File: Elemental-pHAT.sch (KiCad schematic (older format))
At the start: 7 parts

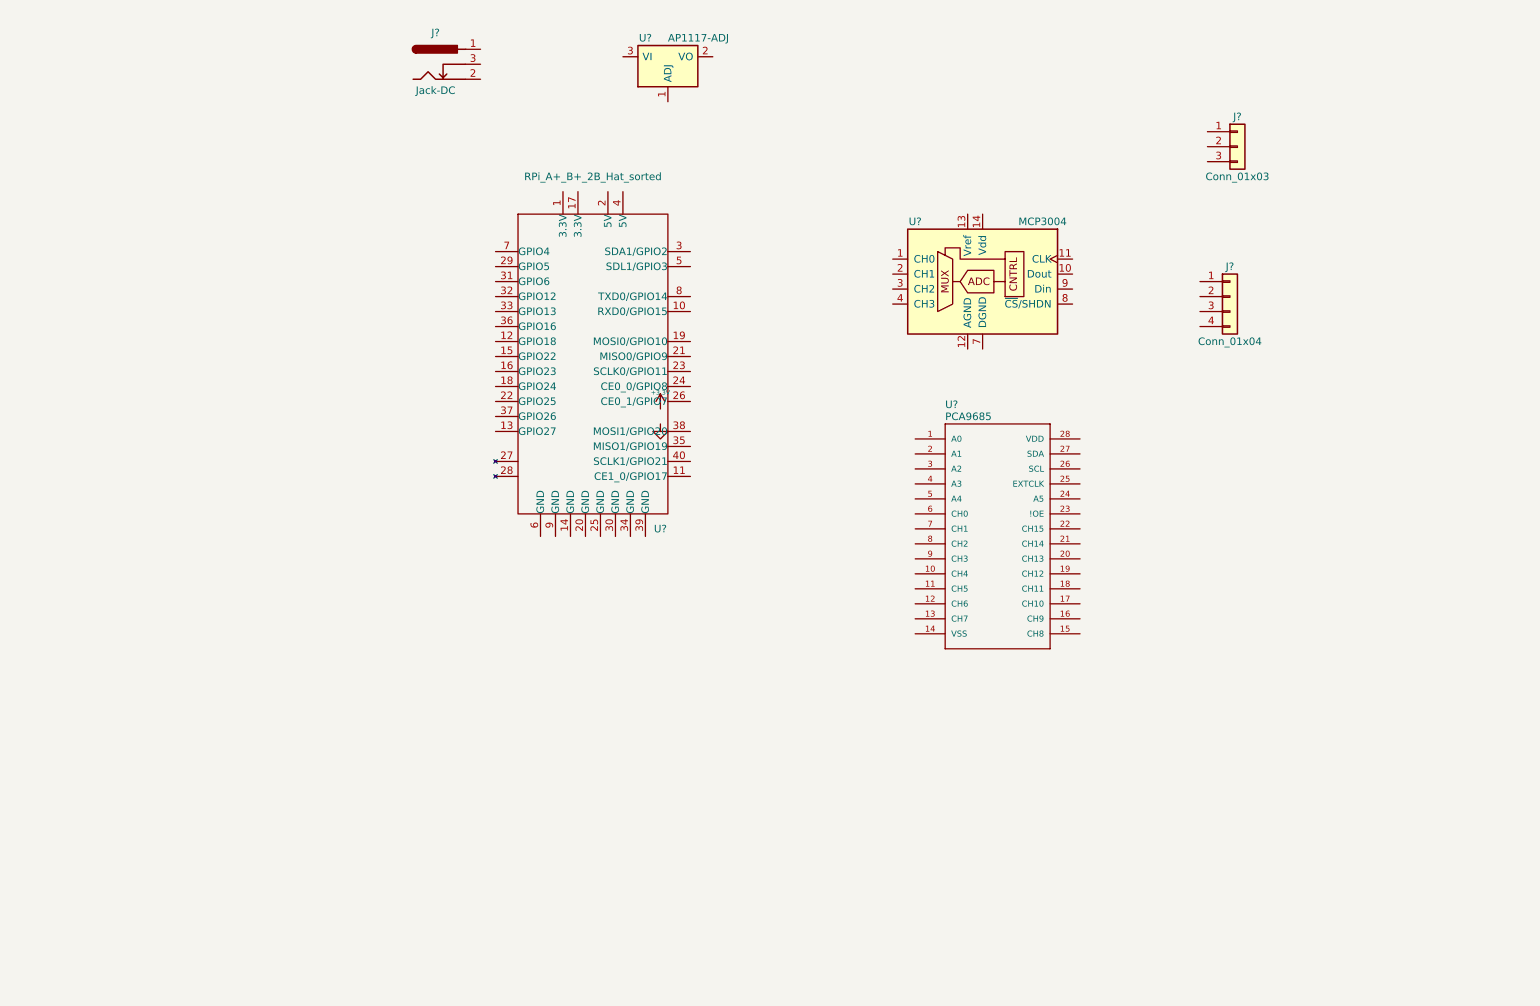
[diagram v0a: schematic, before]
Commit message: conectores añadidos
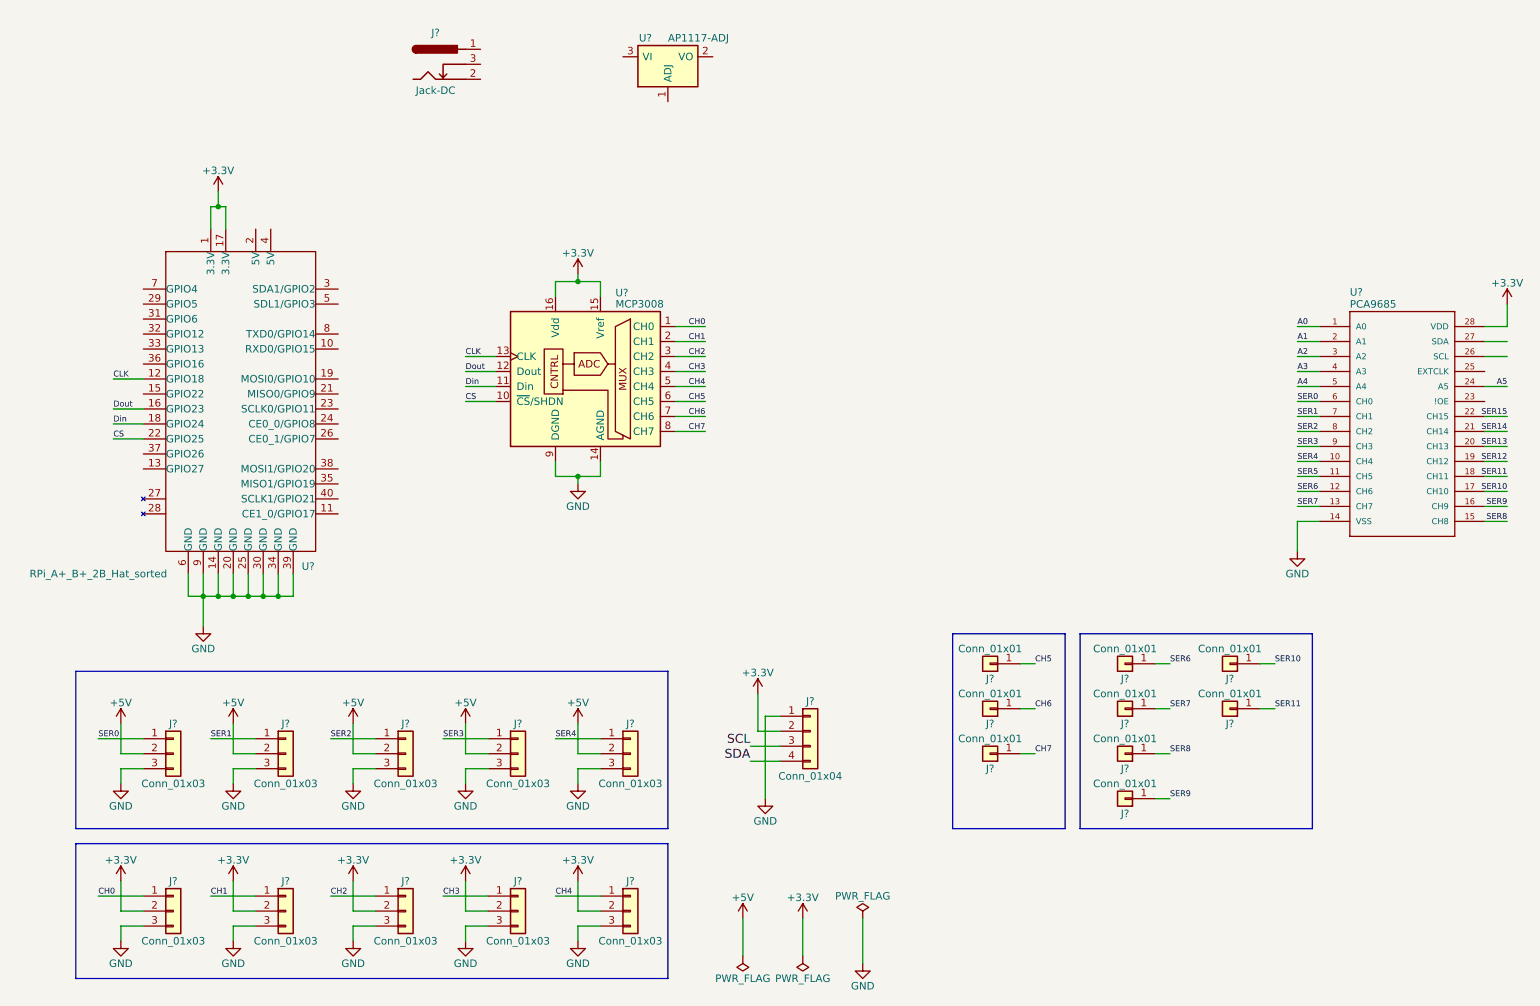
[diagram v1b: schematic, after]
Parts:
- removed U?: MCP3004, symbol MCP3004
- added J? (x9): Conn_01x03, symbol Conn_01x03
- added J? (x9): Conn_01x01, symbol Conn_01x01
- added U?: MCP3008, symbol MCP3008
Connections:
- net +3V3: now also J?.2 (Pin_2), J?.2 (Pin_2), U?.1 (3.3V), U?.17 (3.3V), U?.28 (VDD), J?.2 (Pin_2), J?.2 (Pin_2), J?.2 (Pin_2), J?.2 (Pin_2), U?.15 (Vref), U?.16 (Vdd)
- net GND: now also J?.1 (Pin_1), J?.3 (Pin_3), U?.14 (GND), U?.14 (VSS), U?.20 (GND), U?.25 (GND), U?.30 (GND), U?.34 (GND), U?.39 (GND), U?.6 (GND), U?.9 (GND), J?.3 (Pin_3), J?.3 (Pin_3), J?.3 (Pin_3), J?.3 (Pin_3), J?.3 (Pin_3), J?.3 (Pin_3), J?.3 (Pin_3), J?.3 (Pin_3), J?.3 (Pin_3), U?.14 (AGND), U?.9 (DGND)
- net CLK: now reaches U?.12 (GPIO18)
- net CLK: now also U?.13 (CLK)
- net Dout: now reaches U?.16 (GPIO23)
- net Dout: now also U?.12 (Dout)
- net Din: now reaches U?.18 (GPIO24)
- net Din: now also U?.11 (Din)
- net CS: now reaches U?.22 (GPIO25)
- net CS: now also U?.10 (~CS~/SHDN)
- net A0: now reaches U?.1 (A0)
- net SER4: now reaches U?.10 (CH4)
- net SER4: now also J?.1 (Pin_1)
- net SER5: now reaches U?.11 (CH5)
- net SER6: now reaches U?.12 (CH6)
- net SER6: now also J?.1 (Pin_1)
- net SER7: now reaches U?.13 (CH7)
- net SER7: now also J?.1 (Pin_1)
- net SER8: now reaches U?.15 (CH8)
- net SER8: now also J?.1 (Pin_1)
- net SER9: now reaches U?.16 (CH9)
- net SER9: now also J?.1 (Pin_1)
- net SER10: now reaches U?.17 (CH10)
- net SER10: now also J?.1 (Pin_1)
- net SER11: now reaches U?.18 (CH11)
- net SER11: now also J?.1 (Pin_1)
- net SER12: now reaches U?.19 (CH12)
- net A1: now reaches U?.2 (A1)
- net SER13: now reaches U?.20 (CH13)
- net SER14: now reaches U?.21 (CH14)
- net SER15: now reaches U?.22 (CH15)
- net A5: now reaches U?.24 (A5)
- net A2: now reaches U?.3 (A2)
- net A3: now reaches U?.4 (A3)
- net A4: now reaches U?.5 (A4)
- net SER0: now reaches U?.6 (CH0)
- net SER0: now also J?.1 (Pin_1)
- net SER1: now reaches U?.7 (CH1)
- net SER1: now also J?.1 (Pin_1)
- net SER2: now reaches U?.8 (CH2)
- net SER2: now also J?.1 (Pin_1)
- net SER3: now reaches U?.9 (CH3)
- net SER3: now also J?.1 (Pin_1)
- net CH0: now reaches J?.1 (Pin_1)
- net CH0: now also U?.1 (CH0)
- net SCL: now reaches J?.3 (Pin_3)
- net SDA: now reaches J?.4 (Pin_4)
- new net +5V: J?.2 (Pin_2), J?.2 (Pin_2), J?.2 (Pin_2), J?.2 (Pin_2), J?.2 (Pin_2)
- new net CH1: J?.1 (Pin_1), U?.2 (CH1)
- new net CH2: J?.1 (Pin_1), U?.3 (CH2)
- new net CH3: J?.1 (Pin_1), U?.4 (CH3)
- new net CH4: J?.1 (Pin_1), U?.5 (CH4)
- new net CH5: J?.1 (Pin_1), U?.6 (CH5)
- new net CH6: J?.1 (Pin_1), U?.7 (CH6)
- new net CH7: J?.1 (Pin_1), U?.8 (CH7)
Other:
- moved on the sheet: J?, U?

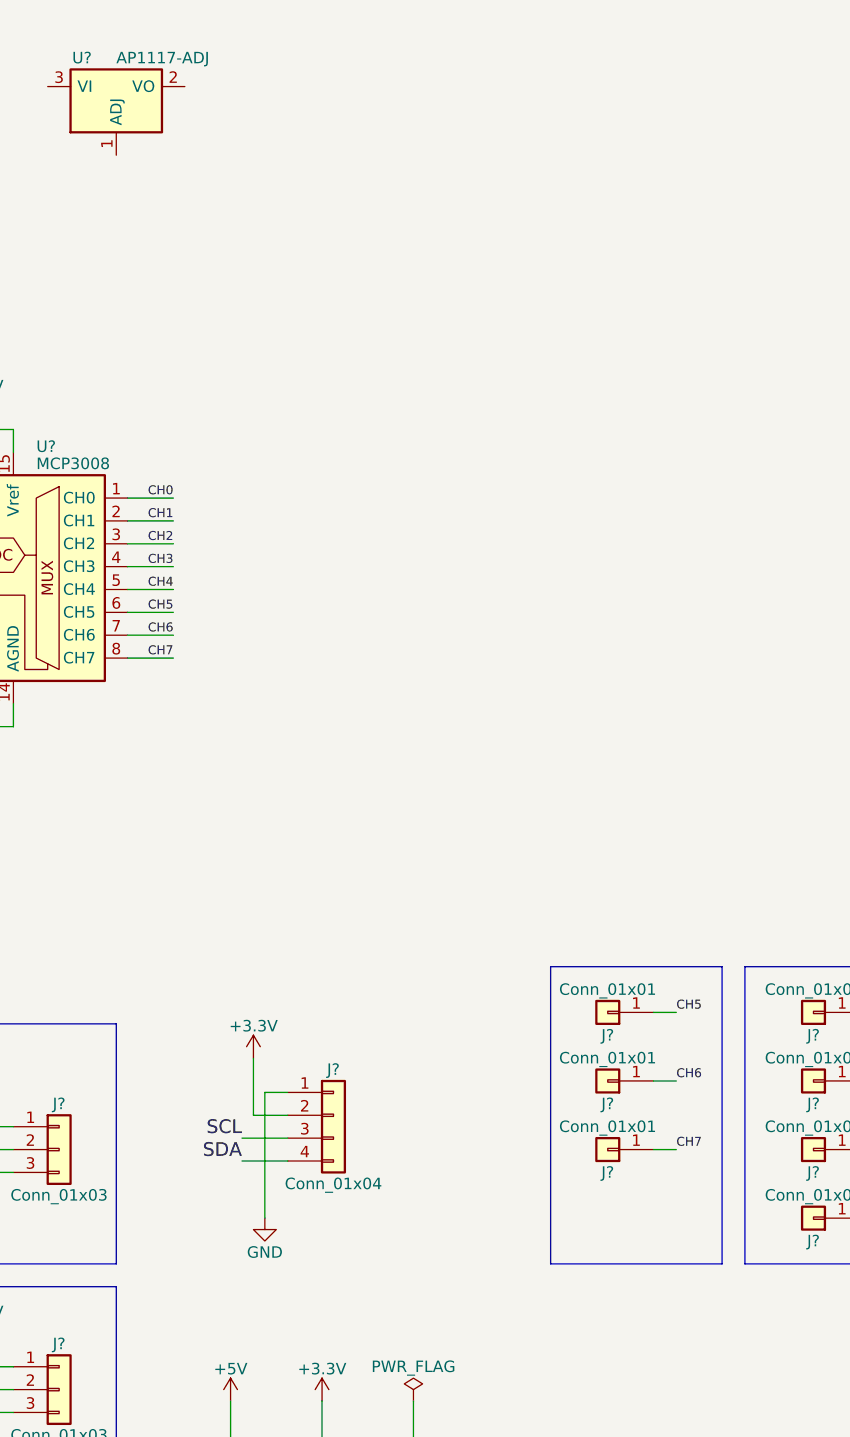
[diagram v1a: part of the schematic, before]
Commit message: Jumpers añadidos
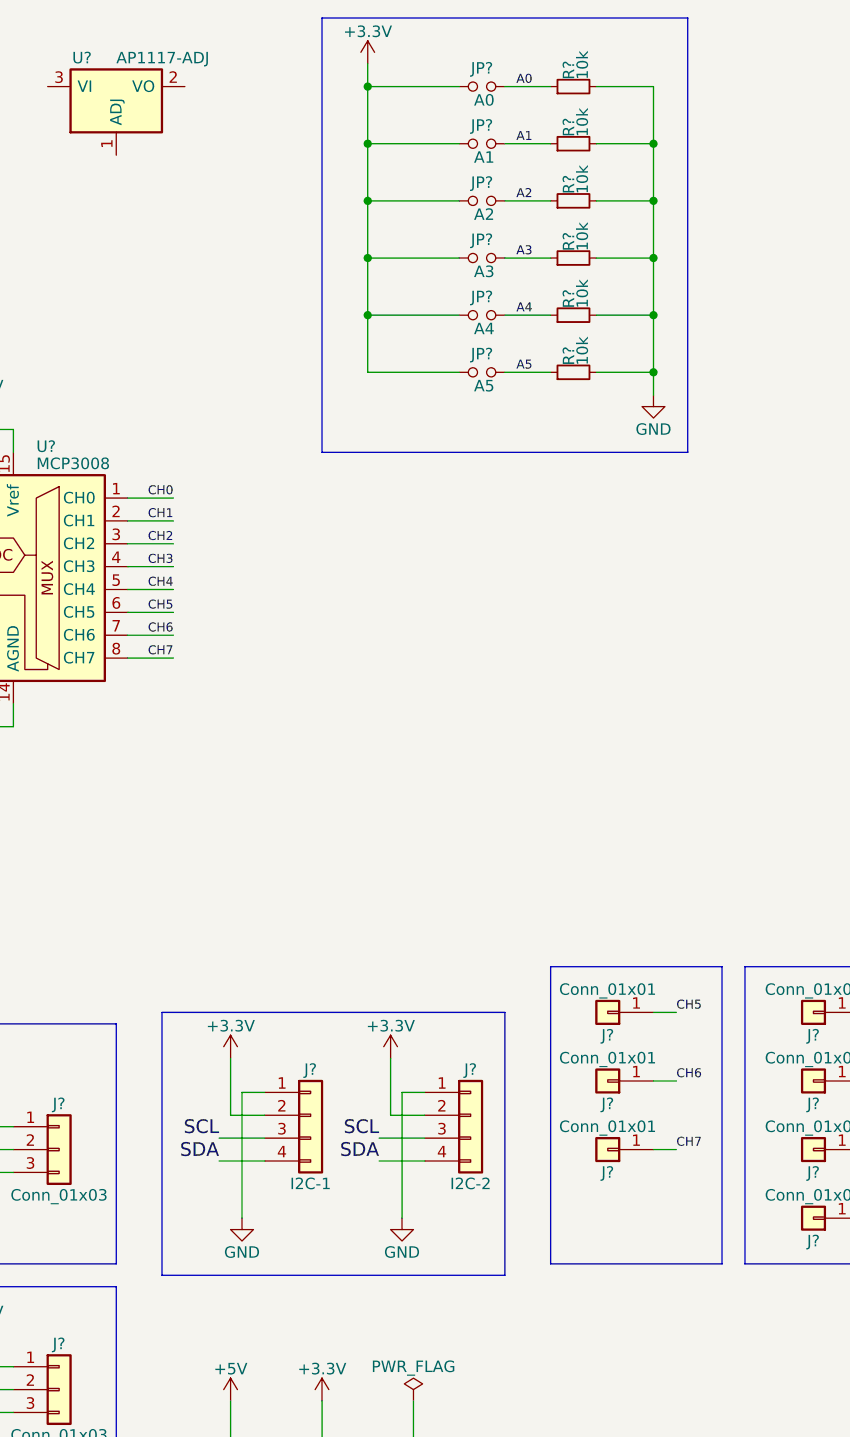
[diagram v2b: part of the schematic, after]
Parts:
- added J?: I2C-2, symbol Conn_01x04
- added JP?: A0, symbol Jumper_NO_Small
- added JP?: A1, symbol Jumper_NO_Small
- added JP?: A2, symbol Jumper_NO_Small
- added JP?: A3, symbol Jumper_NO_Small
- added JP?: A4, symbol Jumper_NO_Small
- added JP?: A5, symbol Jumper_NO_Small
- added R? (x6): 10k, symbol R_Small
- J?: value Conn_01x04 -> I2C-1
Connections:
- net +3V3: now also J?.2 (Pin_2), JP?.1, JP?.1, JP?.1, JP?.1, JP?.1, JP?.1
- net A0: now also JP?.2, R?.1
- net A1: now also JP?.2, R?.1
- net A2: now also JP?.2, R?.1
- net A3: now also JP?.2, R?.1
- net A4: now also JP?.2, R?.1
- net A5: now also JP?.2, R?.1
- net GND: now also J?.1 (Pin_1), R?.2, R?.2, R?.2, R?.2, R?.2, R?.2
- net SCL: now also J?.3 (Pin_3)
- net SDA: now also J?.4 (Pin_4)
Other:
- moved on the sheet: J?

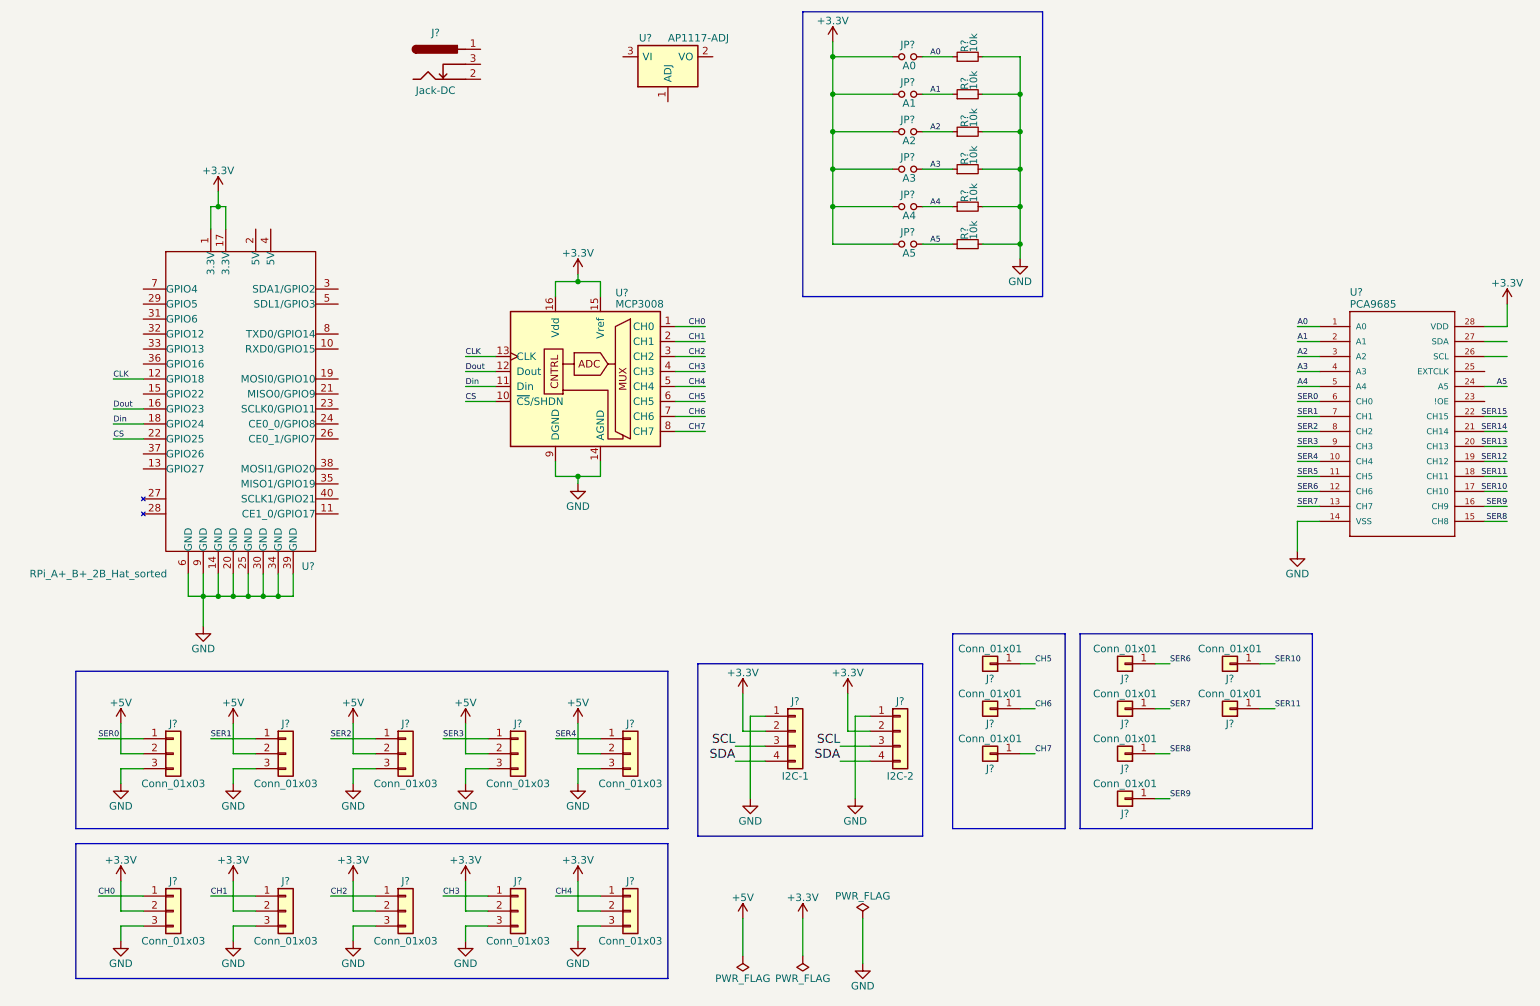
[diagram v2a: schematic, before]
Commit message: Nombres puestos
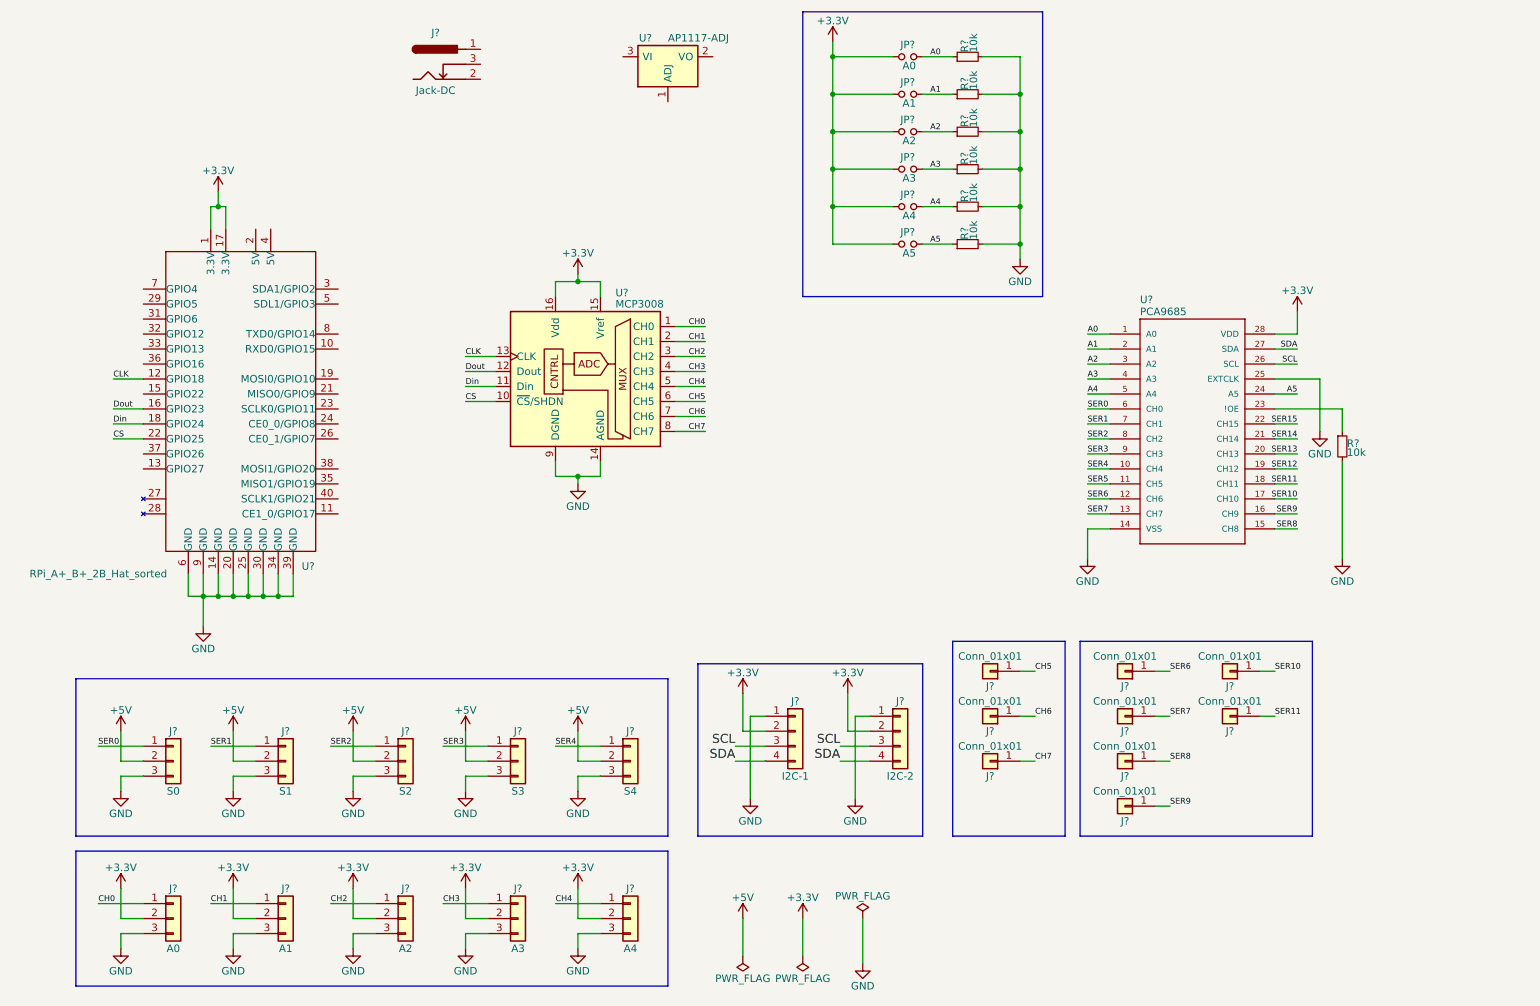
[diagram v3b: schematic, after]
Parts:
- added R?: 10k, symbol R_Small
- J?: value Conn_01x03 -> A0
- J?: value Conn_01x03 -> A1
- J?: value Conn_01x03 -> A2
- J?: value Conn_01x03 -> A3
- J?: value Conn_01x03 -> S0
- J?: value Conn_01x03 -> S1
- J?: value Conn_01x03 -> S2
- J?: value Conn_01x03 -> S3
- J?: value Conn_01x03 -> A4
- J?: value Conn_01x03 -> S4
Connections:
- net GND: now also U?.25 (EXTCLK), R?.2
- net SCL: now also U?.26 (SCL)
- net SDA: now also U?.27 (SDA)
- net at U?.23 (!OE): now also R?.1
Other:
- moved on the sheet: J?, U?
